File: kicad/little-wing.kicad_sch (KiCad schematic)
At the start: 132 parts, among them IC1 AP7335-WG-7, J1 nice!view, J10 rgb, J11 rows, J12 columns, J13 columns, J2 Battery, J3 trackball, J4 rotary, J5 trackball, J6 nice!view, J7 Battery, J8 rgb, J9 rows, SW1 Power, SW2 Reset, SW3 Reset, SW4 Power, U1 nice!nano v2, U2 PMW3610, U3 nice!nano v2

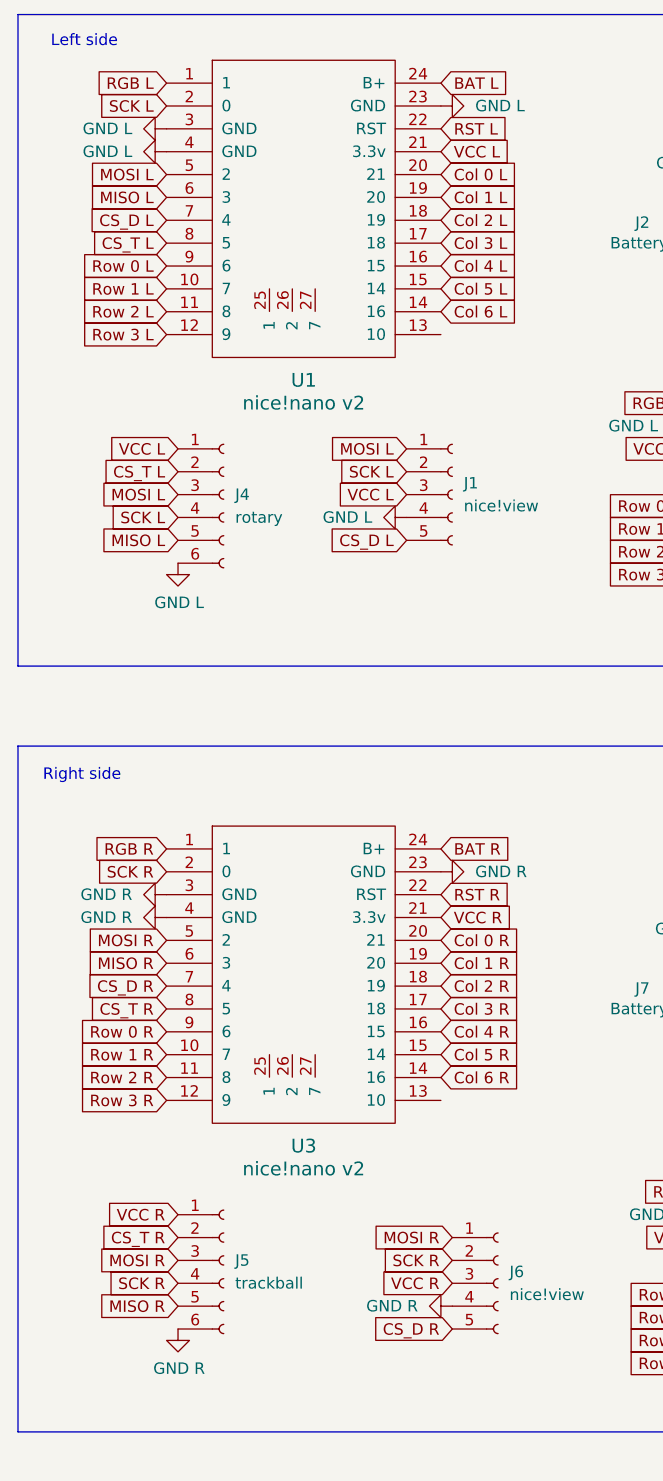
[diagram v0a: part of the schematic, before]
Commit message: Stashig the work
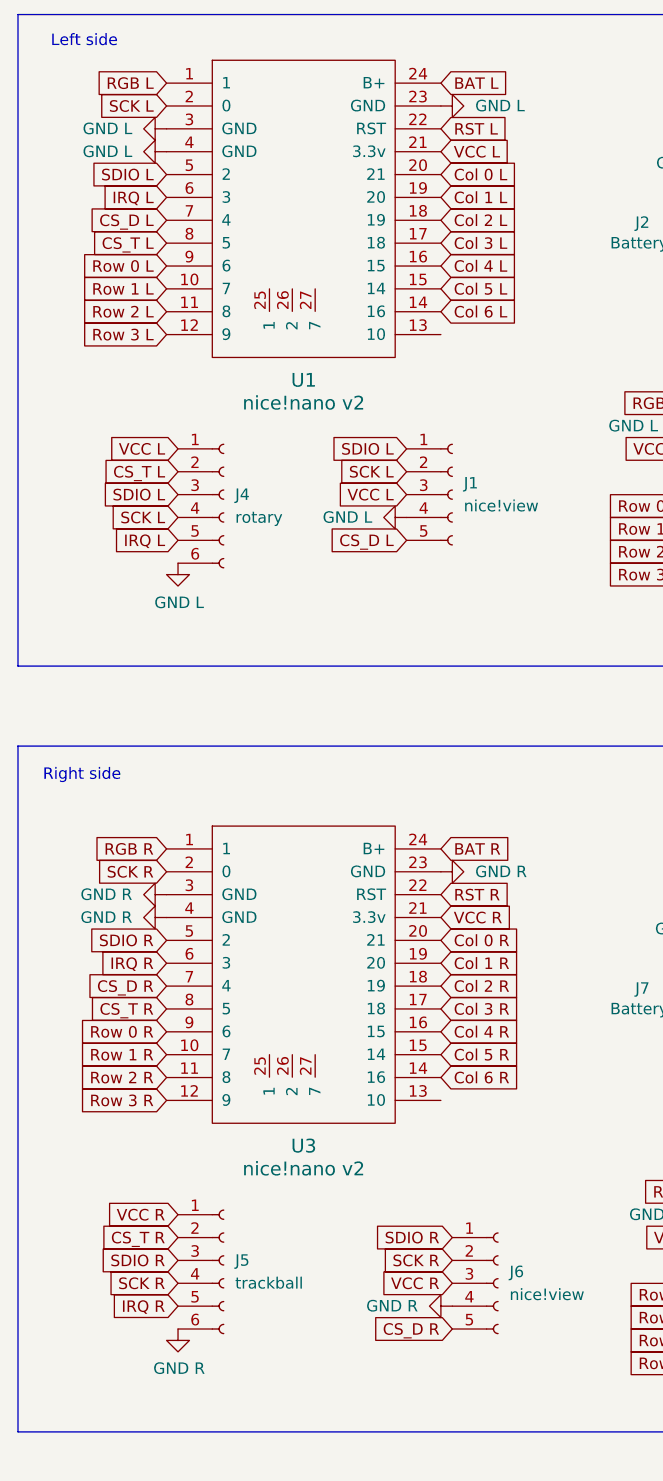
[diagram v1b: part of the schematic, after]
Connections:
- net MISO L renamed IRQ L
- net MISO R renamed IRQ R
- net MOSI L renamed SDIO L
- net MOSI R renamed SDIO R
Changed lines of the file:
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@@
 		)
 	)
-	(global_label "MISO R"
+	(global_label "IRQ R"
 		(shape input)
 		(at 35.56 121.92 180)
@@
 		)
 		(property "Intersheetrefs" "${INTERSHEET_REFS}"
-			(at 25.741 121.92 0)
+			(at 27.1319 121.92 0)
 			(effects
 				(font
@@
 		)
 	)
-	(global_label "MOSI L"
+	(global_label "SDIO L"
 		(shape input)
 		(at 36.83 69.85 180)
@@
 		)
 		(property "Intersheetrefs" "${INTERSHEET_REFS}"
-			(at 27.2529 69.85 0)
+			(at 27.4343 69.85 0)
 			(effects
 				(font
@@
 		)
 	)
-	(global_label "MOSI R"
+	(global_label "SDIO R"
 		(shape input)
 		(at 36.83 154.94 180)
@@
 		)
 		(property "Intersheetrefs" "${INTERSHEET_REFS}"
-			(at 27.011 154.94 0)
+			(at 27.1924 154.94 0)
 			(effects
 				(font
@@
 		)
 	)
-	(global_label "MOSI L"
+	(global_label "SDIO L"
 		(shape input)
 		(at 35.56 34.29 180)
@@
 		)
 		(property "Intersheetrefs" "${INTERSHEET_REFS}"
-			(at 25.9829 34.29 0)
-			(effects
-				(font
-					(size 1.27 1.27)
-				)
-				(justify right)
-				(hide yes)
-			)
-		)
-	)
-	(global_label "MISO L"
+			(at 26.1643 34.29 0)
+			(effects
+				(font
+					(size 1.27 1.27)
+				)
+				(justify right)
+				(hide yes)
+			)
+		)
+	)
+	(global_label "IRQ L"
 		(shape input)
 		(at 35.56 36.83 180)
@@
 		)
 		(property "Intersheetrefs" "${INTERSHEET_REFS}"
-			(at 25.9829 36.83 0)
+			(at 27.3738 36.83 0)
 			(effects
 				(font
@@
 		)
 	)
-	(global_label "MOSI R"
+	(global_label "SDIO R"
 		(shape input)
 		(at 67.31 152.4 180)
@@
 		)
 		(property "Intersheetrefs" "${INTERSHEET_REFS}"
-			(at 57.491 152.4 0)
+			(at 57.6724 152.4 0)
 			(effects
 				(font
@@
 		)
 	)
-	(global_label "MOSI R"
+	(global_label "SDIO R"
 		(shape input)
 		(at 35.56 119.38 180)
@@
 		)
 		(property "Intersheetrefs" "${INTERSHEET_REFS}"
-			(at 25.741 119.38 0)
+			(at 25.9224 119.38 0)
 			(effects
 				(font
@@
 		)
 	)
-	(global_label "MOSI L"
+	(global_label "SDIO L"
 		(shape input)
 		(at 62.23 64.77 180)
@@
 		)
 		(property "Intersheetrefs" "${INTERSHEET_REFS}"
-			(at 52.6529 64.77 0)
+			(at 52.8343 64.77 0)
 			(effects
 				(font
@@
 		)
 	)
-	(global_label "MISO R"
+	(global_label "IRQ R"
 		(shape input)
 		(at 36.83 160.02 180)
@@
 		)
 		(property "Intersheetrefs" "${INTERSHEET_REFS}"
-			(at 27.011 160.02 0)
+			(at 28.4019 160.02 0)
 			(effects
 				(font
@@
 		)
 	)
-	(global_label "MISO L"
+	(global_label "IRQ L"
 		(shape input)
 		(at 36.83 74.93 180)
@@
 		)
 		(property "Intersheetrefs" "${INTERSHEET_REFS}"
-			(at 27.2529 74.93 0)
-			(effects
-				(font
+			(at 28.6438 74.93 0)
+			(effects
+				(font
